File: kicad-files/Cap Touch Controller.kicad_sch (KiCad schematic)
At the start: 37 parts, among them J1 USB_C_Receptacle_USB2.0, J2 8-pin_header, J3 8-pin_header, SW1 SW_Push, U1 ATSAMD21J15B-A, U2 MIC5365-3.3YD5

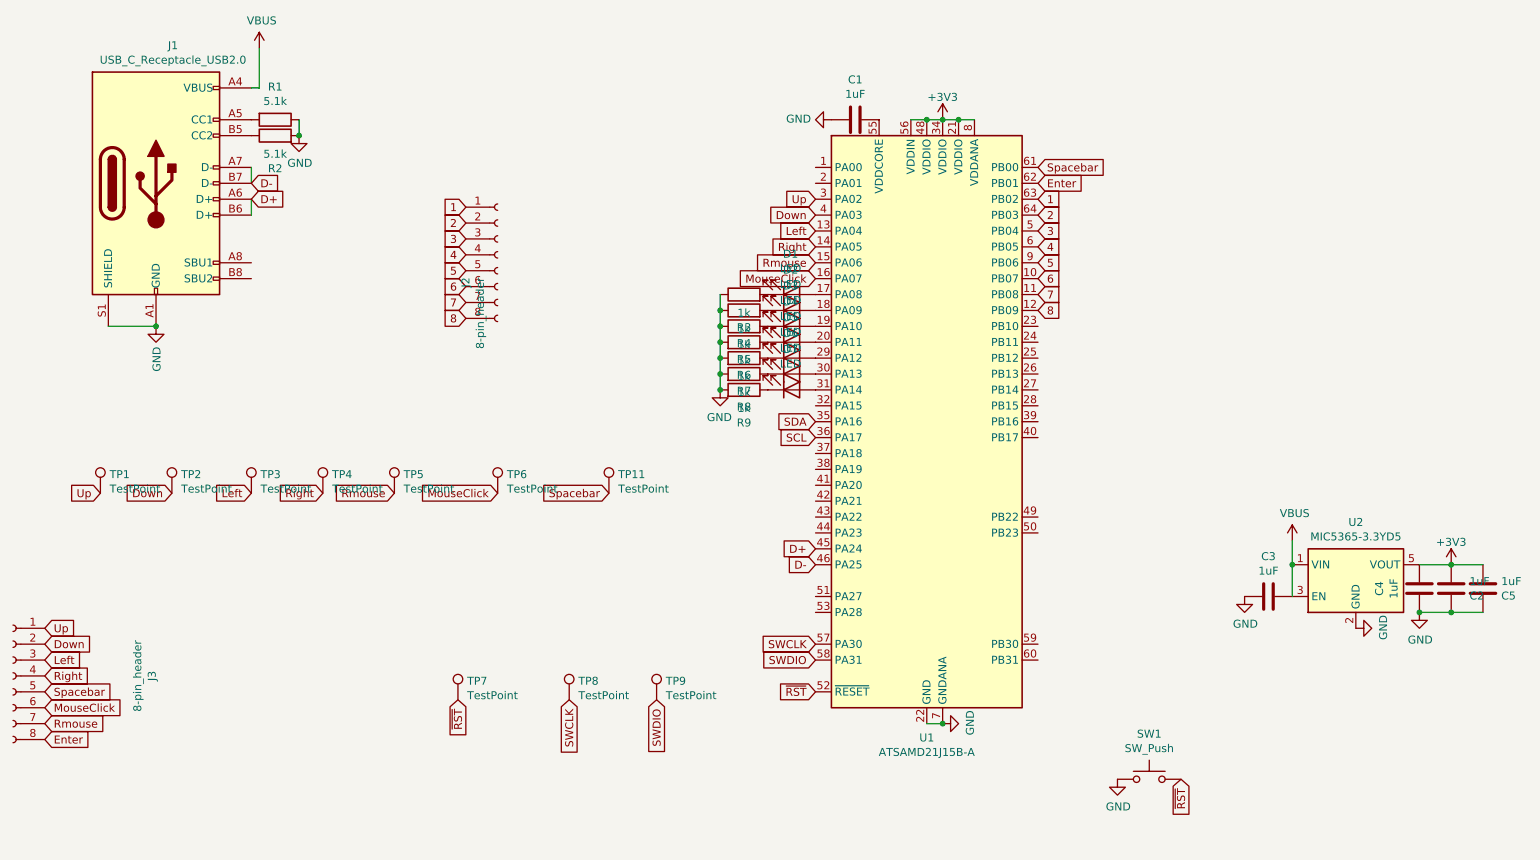
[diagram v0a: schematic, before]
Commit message: Added Files
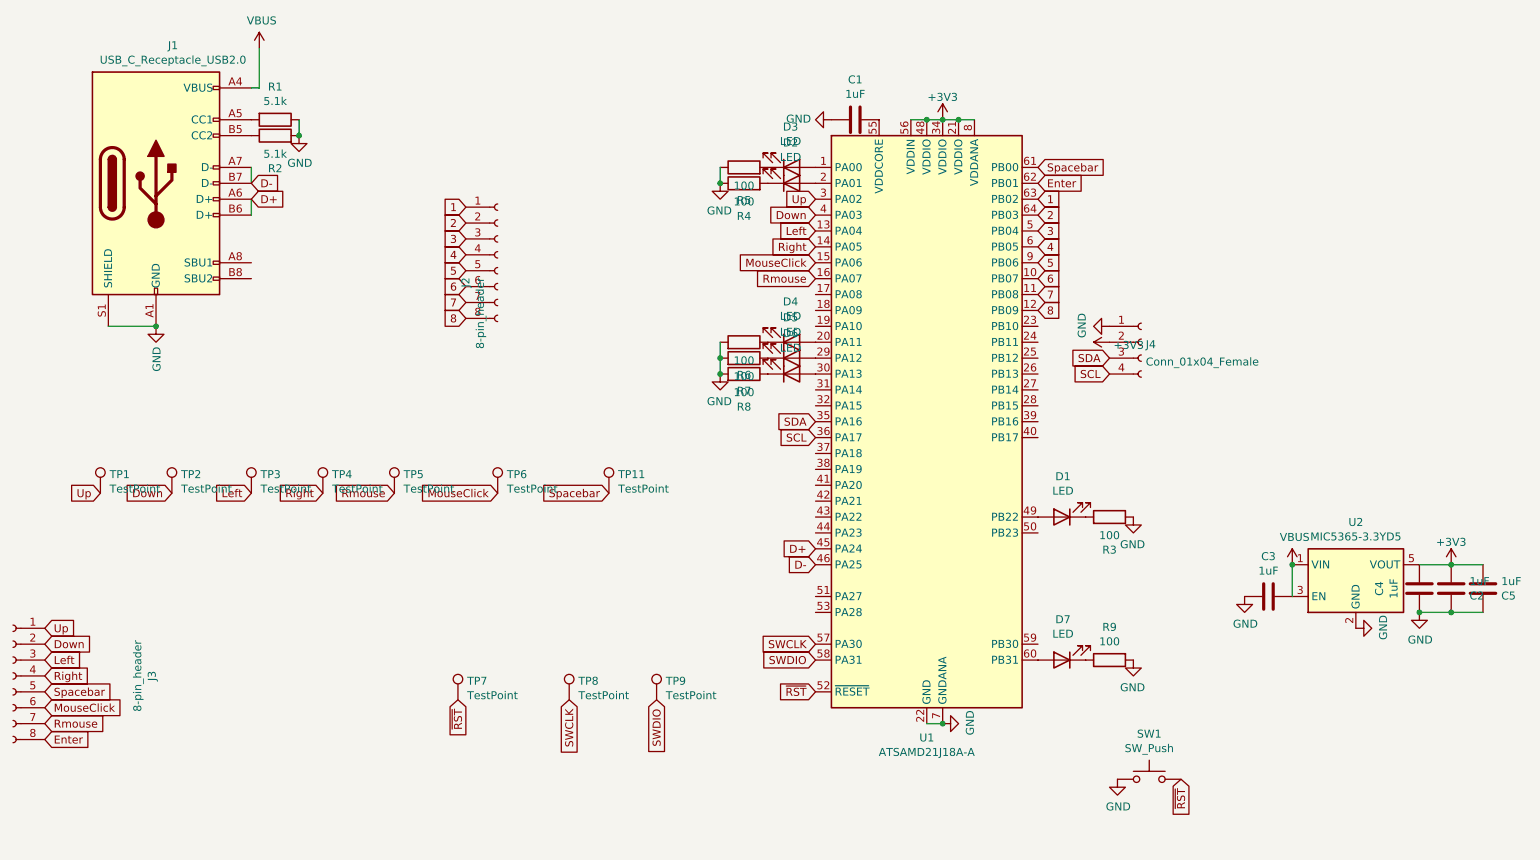
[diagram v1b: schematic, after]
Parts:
- added J4: Conn_01x04_Female, Connector_JST:JST_SH_BM04B-SRSS-TB_1x04-1MP_P1.00mm_Vertical, symbol Connector:Conn_01x04_Female
- R3, R4, R5, R6, R7, R8, R9: value 1k -> 100
- SW1: footprint Button_Switch_SMD:SW_Push_1P1T_NO_6x6mm_H9.5mm -> Button_Switch_SMD:SW_SPST_PTS645
- U1: value ATSAMD21J15B-A -> ATSAMD21J18A-A; symbol MCU_Microchip_SAMD:ATSAMD21J15B-A -> MCU_Microchip_SAMD:ATSAMD21J18A-A
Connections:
- net +3V3: now also J4.2 (Pin_2)
- net GND: now also J4.1 (Pin_1)
- net MouseClick: now also U1.15 (PA06); no longer U1.16 (PA07)
- net Rmouse: now also U1.16 (PA07); no longer U1.15 (PA06)
- net SCL: now also J4.4 (Pin_4)
- net SDA: now also J4.3 (Pin_3)
- net at D1.2 (A): now also U1.49 (PB22); no longer U1.17 (PA08)
- net at U1.1 (PA00): now also D3.2 (A)
- net at U1.18 (PA09): no longer D2.2 (A)
- net at U1.19 (PA10): no longer D3.2 (A)
- net at U1.2 (PA01): now also D2.2 (A)
- net at U1.31 (PA14): no longer D7.2 (A)
- net at U1.60 (PB31): now also D7.2 (A)
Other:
- moved on the sheet: D1, D2, D3, D7, R3, R4, R5, R9

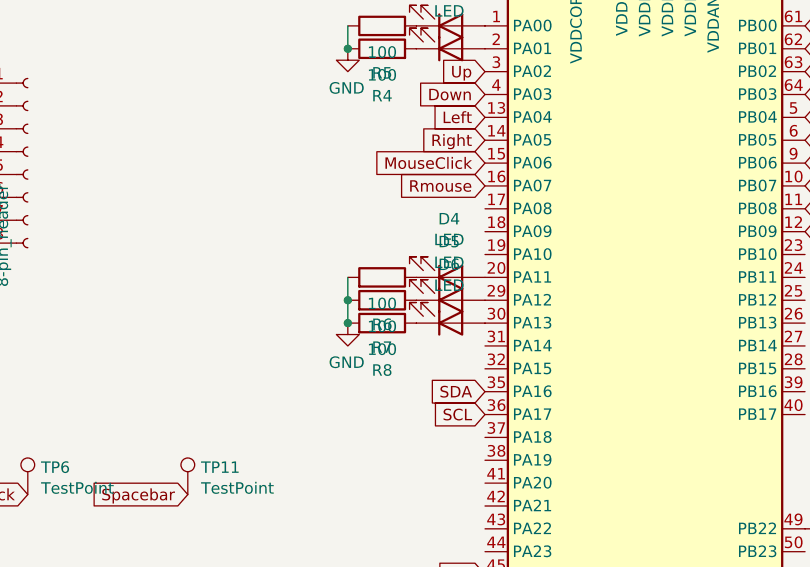
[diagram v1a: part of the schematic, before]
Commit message: Changed files
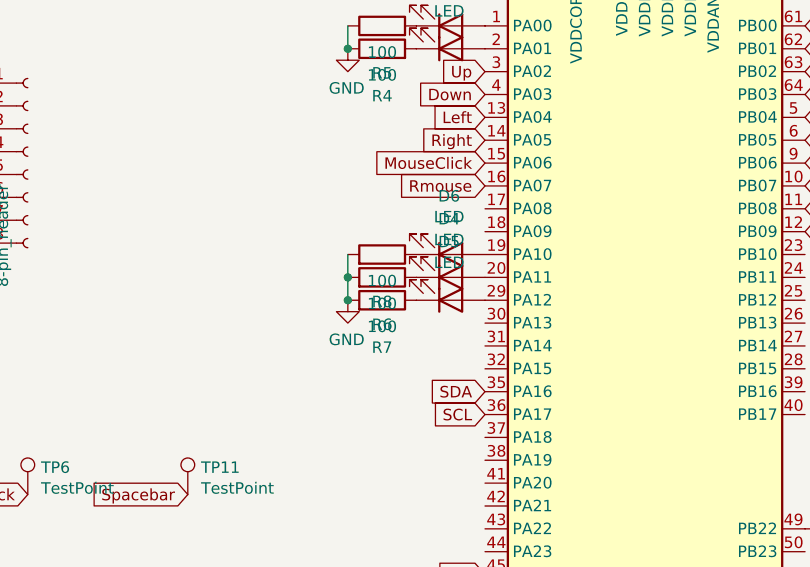
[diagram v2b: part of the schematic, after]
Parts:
- J4: footprint Connector_JST:JST_SH_BM04B-SRSS-TB_1x04-1MP_P1.00mm_Vertical -> Connector_JST:JST_SH_SM04B-SRSS-TB_1x04-1MP_P1.00mm_Horizontal
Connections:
- net at U1.19 (PA10): now also D6.2 (A)
- net at U1.30 (PA13): no longer D6.2 (A)
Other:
- moved on the sheet: D6, R8
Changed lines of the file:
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@@
   (junction (at 194.31 29.21) (diameter 0) (color 0 0 0 0)
   )
-  (junction (at 158.75 69.85) (diameter 0) (color 0 0 0 0)
-  )
   (junction (at 158.75 39.37) (diameter 0) (color 0 0 0 0)
   )
@@
   (junction (at 196.85 29.21) (diameter 0) (color 0 0 0 0)
   )
+  (junction (at 158.75 64.77) (diameter 0) (color 0 0 0 0)
+  )
   (junction (at 158.75 67.31) (diameter 0) (color 0 0 0 0)
   )
@@
     (stroke (width 0) (type default) (color 0 0 0 0))
   )
-  (wire (pts (xy 158.75 67.31) (xy 158.75 69.85))
+  (wire (pts (xy 158.75 64.77) (xy 158.75 67.31))
     (stroke (width 0) (type default) (color 0 0 0 0))
   )
@@
     (stroke (width 0) (type default) (color 0 0 0 0))
   )
-  (wire (pts (xy 158.75 64.77) (xy 158.75 67.31))
+  (wire (pts (xy 158.75 62.23) (xy 158.75 64.77))
     (stroke (width 0) (type default) (color 0 0 0 0))
   )
@@
     (pin "2")
   )
-  (symbol (lib_id "Device:LED") (at 170.18 69.85 0) (mirror x) (unit 1)
-    (in_bom yes) (on_board yes)
-    (property "Reference" "D6" (id 0) (at 170.0022 63.373 0))
-    (property "Value" "LED" (id 1) (at 170.0022 65.6844 0))
-    (property "Footprint" "LED_SMD:LED_0603_1608Metric_Castellated" (id 2) (at 170.18 69.85 0)
-      (effects (font (size 1.27 1.27)) hide)
-    )
-    (property "Datasheet" "~" (id 3) (at 170.18 69.85 0)
+  (symbol (lib_id "Device:LED") (at 170.18 62.23 0) (mirror x) (unit 1)
+    (in_bom yes) (on_board yes)
+    (property "Reference" "D6" (id 0) (at 170.0022 55.753 0))
+    (property "Value" "LED" (id 1) (at 170.0022 58.0644 0))
+    (property "Footprint" "LED_SMD:LED_0603_1608Metric_Castellated" (id 2) (at 170.18 62.23 0)
+      (effects (font (size 1.27 1.27)) hide)
+    )
+    (property "Datasheet" "~" (id 3) (at 170.18 62.23 0)
       (effects (font (size 1.27 1.27)) hide)
     )
@@
     (pin "1")
   )
-  (symbol (lib_id "power:GND") (at 158.75 69.85 0) (mirror y) (unit 1)
-    (in_bom yes) (on_board yes)
-    (property "Reference" "#PWR0101" (id 0) (at 158.75 76.2 0)
-      (effects (font (size 1.27 1.27)) hide)
-    )
-    (property "Value" "GND" (id 1) (at 158.623 74.2442 0))
-    (property "Footprint" "" (id 2) (at 158.75 69.85 0)
-      (effects (font (size 1.27 1.27)) hide)
-    )
-    (property "Datasheet" "" (id 3) (at 158.75 69.85 0)
+  (symbol (lib_id "power:GND") (at 158.75 67.31 0) (mirror y) (unit 1)
+    (in_bom yes) (on_board yes)
+    (property "Reference" "#PWR0101" (id 0) (at 158.75 73.66 0)
+      (effects (font (size 1.27 1.27)) hide)
+    )
+    (property "Value" "GND" (id 1) (at 158.623 71.7042 0))
+    (property "Footprint" "" (id 2) (at 158.75 67.31 0)
+      (effects (font (size 1.27 1.27)) hide)
+    )
+    (property "Datasheet" "" (id 3) (at 158.75 67.31 0)
       (effects (font (size 1.27 1.27)) hide)
     )
@@
     (pin "1")
   )
-  (symbol (lib_id "Device:R") (at 162.56 69.85 270) (mirror x) (unit 1)
-    (in_bom yes) (on_board yes)
-    (property "Reference" "R8" (id 0) (at 162.56 75.1078 90))
-    (property "Value" "100" (id 1) (at 162.56 72.7964 90))
-    (property "Footprint" "Resistor_SMD:R_0603_1608Metric_Pad0.98x0.95mm_HandSolder" (id 2) (at 162.56 71.628 90)
-      (effects (font (size 1.27 1.27)) hide)
-    )
-    (property "Datasheet" "~" (id 3) (at 162.56 69.85 0)
+  (symbol (lib_id "Device:R") (at 162.56 62.23 270) (mirror x) (unit 1)
+    (in_bom yes) (on_board yes)
+    (property "Reference" "R8" (id 0) (at 162.56 67.4878 90))
+    (property "Value" "100" (id 1) (at 162.56 65.1764 90))
+    (property "Footprint" "Resistor_SMD:R_0603_1608Metric_Pad0.98x0.95mm_HandSolder" (id 2) (at 162.56 64.008 90)
+      (effects (font (size 1.27 1.27)) hide)
+    )
+    (property "Datasheet" "~" (id 3) (at 162.56 62.23 0)
       (effects (font (size 1.27 1.27)) hide)
     )
@@
       (effects (font (size 1.27 1.27)) (justify left))
     )
-    (property "Footprint" "Connector_JST:JST_SH_BM04B-SRSS-TB_1x04-1MP_P1.00mm_Vertical" (id 2) (at 226.06 64.77 0)
+    (property "Footprint" "Connector_JST:JST_SH_SM04B-SRSS-TB_1x04-1MP_P1.00mm_Horizontal" (id 2) (at 226.06 64.77 0)
       (effects (font (size 1.27 1.27)) hide)
     )
@@
     )
     (path "/b557b950-76ec-4fce-9578-1142ee4ce755"
-      (reference "J4") (unit 1) (value "Conn_01x04_Female") (footprint "Connector_JST:JST_SH_BM04B-SRSS-TB_1x04-1MP_P1.00mm_Vertical")
+      (reference "J4") (unit 1) (value "Conn_01x04_Female") (footprint "Connector_JST:JST_SH_SM04B-SRSS-TB_1x04-1MP_P1.00mm_Horizontal")
     )
     (path "/00000000-0000-0000-0000-000061a16f89"
